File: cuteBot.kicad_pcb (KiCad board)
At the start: 2 copper layers, 39.9 x 39.9 mm, 67 parts, among them P1 USB_A, P2 BAT+, P3 BAT-, P4 MOTOR_A, P5 MOTOR_B, P6 CONN_02X03, Q1 S8050, SW1 SW_SPDT, SW2 SW_Push, SW3 SW_Push, U1 ATMEGA32U4-MU, U2 TP4056, U3 FS312F-G, U4 FS8205, U5 MT3608, U6 DRV8833RTY, U7 JDY-08, U8 MIC5219-3.3, Y1 16MHz

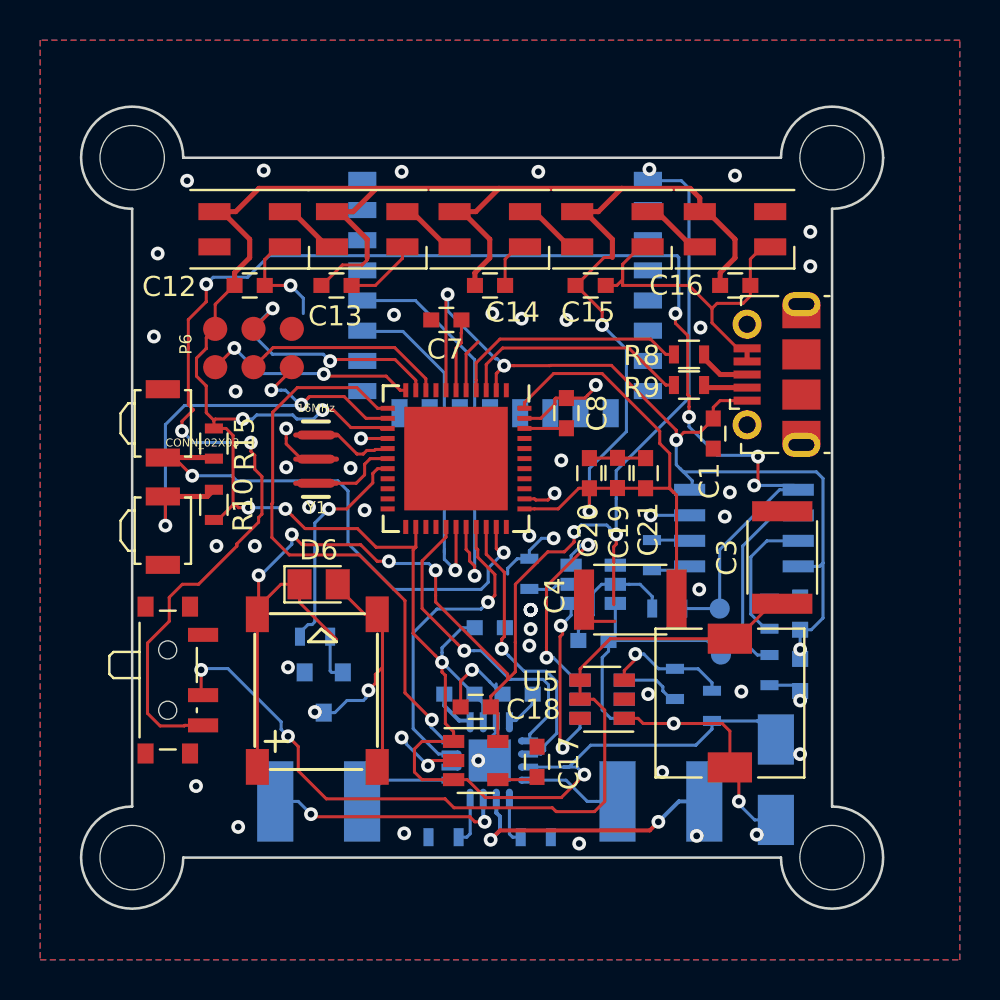
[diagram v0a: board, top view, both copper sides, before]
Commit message: Serigrafía terminada
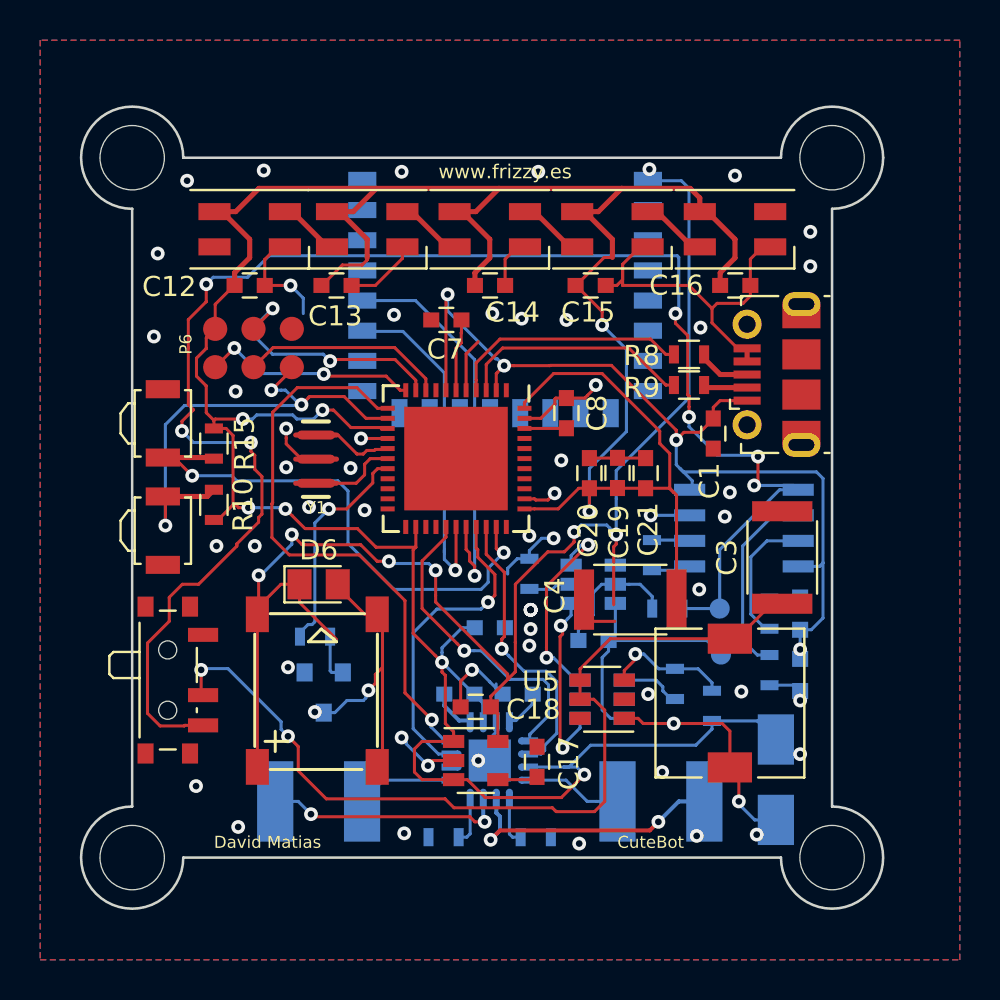
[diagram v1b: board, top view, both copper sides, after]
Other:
- board text added: "+"
- board text added: "-"
- board text added: "CuteBot"
- board text added: "David Matias"
- board text added: "www.frizzy.es"
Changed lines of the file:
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@@
   (general
     (thickness 1.6)
-    (drawings 12)
+    (drawings 17)
     (tracks 863)
     (zones 0)
@@
     (pad_to_paste_clearance -0.04)
     (aux_axis_origin 0 0)
-    (visible_elements FFFDFF7F)
+    (visible_elements FFFFFF7F)
     (pcbplotparams
       (layerselection 0x3ffff_80000001)
@@
       (effects (font (size 0.6096 0.6096) (thickness 0.127)))
     )
-    (fp_text value CONN_02X03 (at -2.54 4.7752) (layer F.SilkS)
+    (fp_text value CONN_02X03 (at -2.54 4.7752) (layer F.SilkS) hide
       (effects (font (size 0.4 0.4) (thickness 0.1)))
     )
@@
       (at (xyz 0 0 0))
       (scale (xyz 1 1 1))
+      (rotate (xyz 0 0 0))
+    )
+    (model ${KISYS3DMOD}/Housings_SOIC.3dshapes/SOIJ-8_5.3x5.3mm_Pitch1.27mm.wrl
+      (at (xyz 0 0 0))
+      (scale (xyz 0.8 0.9 0.8))
       (rotate (xyz 0 0 0))
     )
@@
       (effects (font (size 0.4 0.4) (thickness 0.1)) (justify mirror))
     )
-    (fp_text user %R (at 0 2.5 270) (layer B.Fab)
+    (fp_text user %R (at 0.127 0.127 270) (layer B.Fab)
       (effects (font (size 1 1) (thickness 0.15)) (justify mirror))
     )
@@
       (rotate (xyz 0 0 0))
     )
+    (model ${KISYS3DMOD}/Connectors_USB.3dshapes/USB_Micro-B_Molex_47346-0001.wrl
+      (at (xyz 0 0 0))
+      (scale (xyz 1 1 1))
+      (rotate (xyz 0 0 0))
+    )
   )
   (module Connectors_TestPoints:Test_Point_Pad_d1.0mm (layer B.Cu)
@@
     (tags "test point SMD pad")
     (attr virtual)
-    (fp_text reference P2 (at 0 1.448) (layer B.SilkS)
+    (fp_text reference P2 (at 0 1.448) (layer B.SilkS) hide
       (effects (font (size 1 1) (thickness 0.15)) (justify mirror))
     )
@@
     (tags "test point SMD pad")
     (attr virtual)
-    (fp_text reference P3 (at 0 1.448) (layer B.SilkS)
+    (fp_text reference P3 (at 0 1.448) (layer B.SilkS) hide
       (effects (font (size 1 1) (thickness 0.15)) (justify mirror))
     )
@@
     (tags "resistor 0603")
     (attr smd)
-    (fp_text reference R2 (at 0.9405 1.3335 270) (layer B.SilkS)
+    (fp_text reference R2 (at 1.004 1.397 270) (layer B.SilkS)
       (effects (font (size 1 1) (thickness 0.15)) (justify mirror))
     )
@@
     (tags "resistor 0603")
     (attr smd)
-    (fp_text reference R3 (at -0.9525 -0.8255 90) (layer B.SilkS)
+    (fp_text reference R3 (at 2.8575 -0.0635 90) (layer B.SilkS)
       (effects (font (size 1 1) (thickness 0.15)) (justify mirror))
     )
@@
     (pad 17 smd rect (at 0 0 90) (size 2.1 2.1) (layers B.Cu B.Paste B.Mask)
       (net 4 GND) (solder_paste_margin_ratio -0.2))
+    (model ${KISYS3DMOD}/Package_DFN_QFN.3dshapes/MLPQ-16-1EP_4x4mm_P0.65mm_EP2.8x2.8mm.step
+      (at (xyz 0 0 0))
+      (scale (xyz 1 1 1))
+      (rotate (xyz 0 0 0))
+    )
   )
   (module JDY-08:JDY-08 (layer B.Cu)
@@
       (effects (font (size 0.6096 0.6096) (thickness 0.127)))
     )
-    (fp_text value 16MHz (at 2.54 0 -180) (layer F.SilkS)
+    (fp_text value 16MHz (at 2.54 0 180) (layer F.SilkS) hide
       (effects (font (size 0.4 0.4) (thickness 0.1)))
     )
@@
     (pad 3 smd oval (at 1.19888 0 90) (size 0.44958 1.905) (layers F.Cu F.Paste F.Mask)
       (net 90 "Net-(U1-Pad16)") (solder_mask_margin 0.1016))
+    (model "${KISYS3DMOD}/Modelos 3D descargados/Oscilador.wrl"
+      (offset (xyz -1.6 0.7 0))
+      (scale (xyz 0.4 0.4 0.4))
+      (rotate (xyz -90 0 0))
+    )
   )
   (module TO_SOT_Packages_SMD:SOT-23 (layer B.Cu)
@@
       (effects (font (size 0.4 0.4) (thickness 0.1)) (justify mirror))
     )
-    (fp_text user %R (at 0.508 0.254 180) (layer B.Fab)
+    (fp_text user %R (at -0.0475 -0.0025 180) (layer B.Fab)
       (effects (font (size 0.5 0.5) (thickness 0.075)) (justify mirror))
     )
@@
     (pad 1 np_thru_hole circle (at 0 0) (size 3.2 3.2) (drill 3.2) (layers *.Cu *.Mask))
   )
+  (gr_text www.frizzy.es (at 139.954 118.3005) (layer F.SilkS)
+    (effects (font (size 0.7 0.7) (thickness 0.127)))
+  )
+  (gr_text CuteBot (at 147.193 151.638) (layer F.SilkS)
+    (effects (font (size 0.6 0.6) (thickness 0.127)))
+  )
+  (gr_text "David Matias" (at 128.143 151.638) (layer F.SilkS)
+    (effects (font (size 0.6 0.6) (thickness 0.127)))
+  )
+  (gr_text - (at 151.892 142.6845) (layer B.SilkS)
+    (effects (font (size 0.6 0.6) (thickness 0.127)))
+  )
+  (gr_text + (at 151.892 139.192) (layer B.SilkS)
+    (effects (font (size 0.6 0.6) (thickness 0.127)))
+  )
   (gr_line (start 156.21 135.636) (end 121.412 135.636) (layer Dwgs.User) (width 0.127))
